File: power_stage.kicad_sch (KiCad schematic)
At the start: 57 parts, among them J2 red_terminal, J3 4 mm terminal, J4 4 mm terminal, J5 black terminal, Q3 FQP19N20C, Q4 FQP19N20C, Q5 FQP19N20C, Q6 FQP19N20C, U13 TLV9062, U3 NCS21802, U4 NCS21802, U5 TLV9062, U6 TLV9062, U7 LMT84LPM

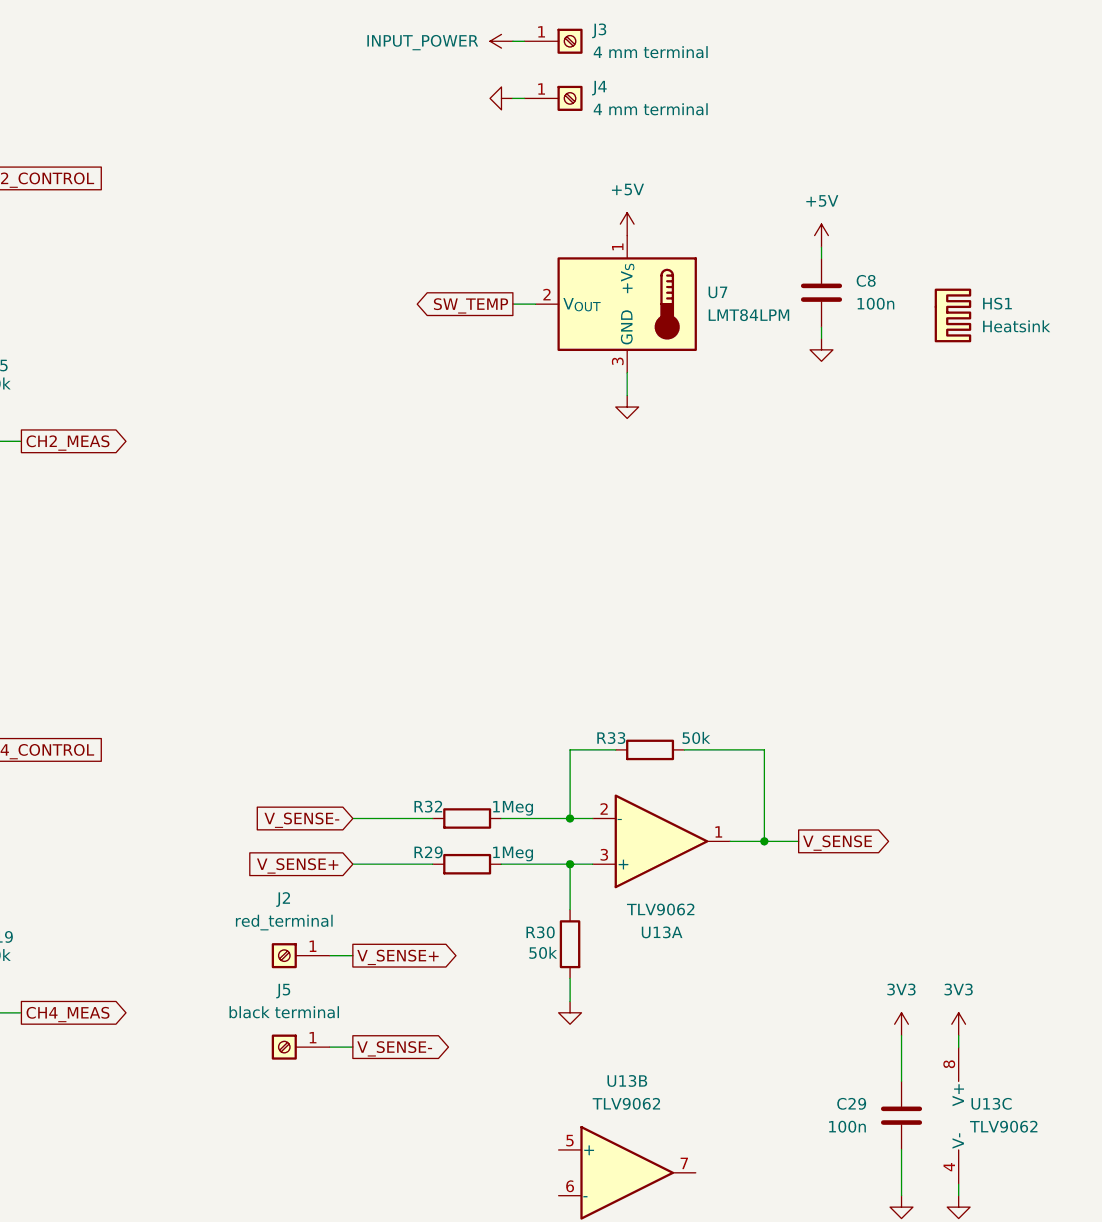
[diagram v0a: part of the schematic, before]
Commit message: aesthetics.
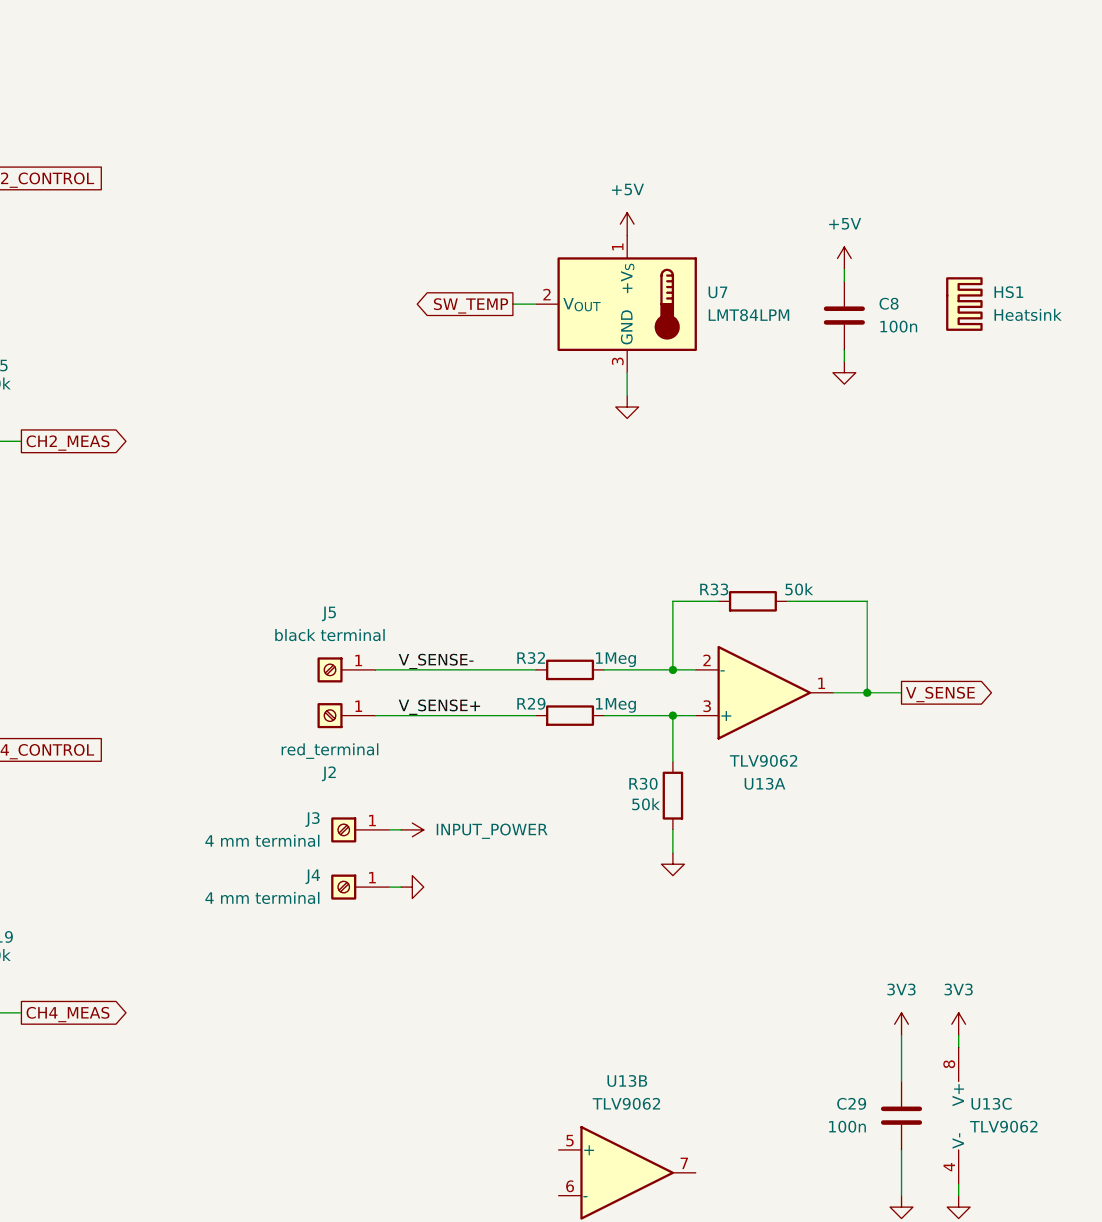
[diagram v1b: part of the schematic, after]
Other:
- moved on the sheet: C8, HS1, J2, J3, J4, J5, R29, R30, R32, R33, U13A
